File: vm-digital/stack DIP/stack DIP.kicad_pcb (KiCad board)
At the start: 2 copper layers, 20.3 x 39.1 mm, 7 parts, among them J1 Conn_01x11_Pin, J2 Conn_01x11_Pin, U1 74LS151, U2 74LS151, U3 74LS151, U4 74LS151, U5 74LS151

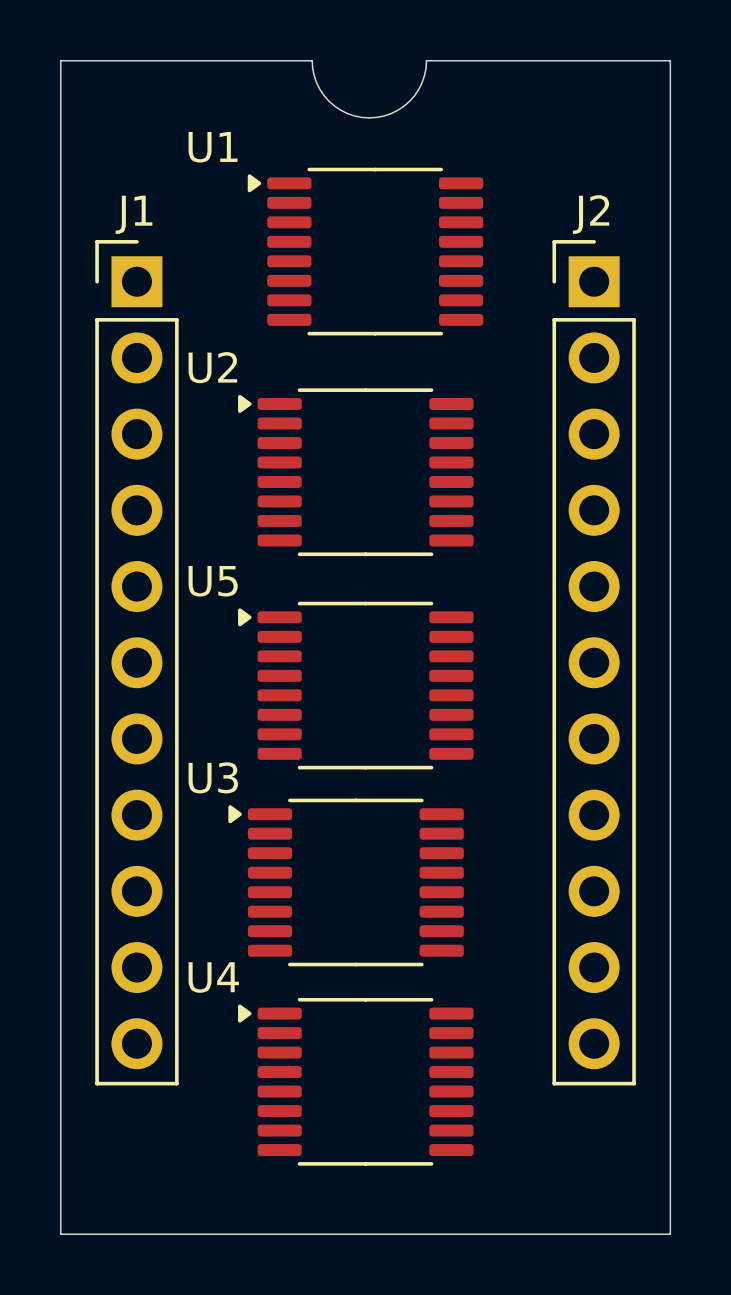
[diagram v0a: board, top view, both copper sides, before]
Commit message: stack-dip
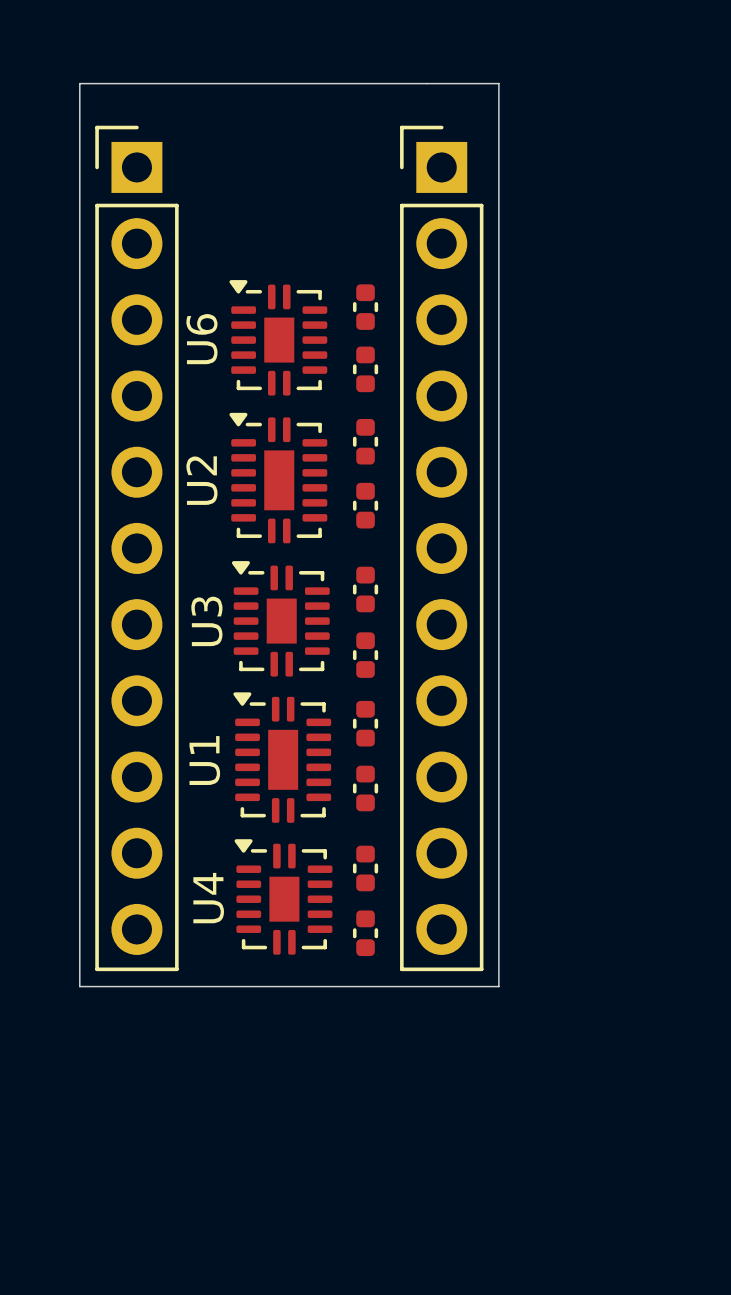
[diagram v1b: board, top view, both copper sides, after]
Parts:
- removed U5: 74LS151, Package_SO:TSSOP-16_4.4x5mm_P0.65mm
- added C1: C_Small, Capacitor_SMD:C_0402_1005Metric, F.Cu at (160.0, 68.2)
- added C10: C_Small, Capacitor_SMD:C_0402_1005Metric, F.Cu at (160.0, 77.6)
- added C2: C_Small, Capacitor_SMD:C_0402_1005Metric, F.Cu at (160.0, 70.2)
- added C3: C_Small, Capacitor_SMD:C_0402_1005Metric, F.Cu at (160.0, 72.6)
- added C4: C_Small, Capacitor_SMD:C_0402_1005Metric, F.Cu at (160.0, 74.8)
- added C5: C_Small, Capacitor_SMD:C_0402_1005Metric, F.Cu at (160.0, 89.0)
- added C6: C_Small, Capacitor_SMD:C_0402_1005Metric, F.Cu at (160.0, 86.9)
- added C7: C_Small, Capacitor_SMD:C_0402_1005Metric, F.Cu at (160.0, 84.2)
- added C8: C_Small, Capacitor_SMD:C_0402_1005Metric, F.Cu at (160.0, 82.0)
- added C9: C_Small, Capacitor_SMD:C_0402_1005Metric, F.Cu at (160.0, 79.8)
- added U6: 7408, Package_DFN_QFN:DHVQFN-14-1EP_2.5x3mm_P0.5mm_EP1x1.5mm, F.Cu at (157.1, 69.3)
- U1: value 74LS151 -> 74LS157; footprint Package_SO:TSSOP-16_4.4x5mm_P0.65mm -> Package_DFN_QFN:DHVQFN-16-1EP_2.5x3.5mm_P0.5mm_EP1x2mm
- U2: footprint Package_SO:TSSOP-16_4.4x5mm_P0.65mm -> Package_DFN_QFN:DHVQFN-16-1EP_2.5x3.5mm_P0.5mm_EP1x2mm
- U3, U4: value 74LS151 -> 74HC74; footprint Package_SO:TSSOP-16_4.4x5mm_P0.65mm -> Package_DFN_QFN:DHVQFN-14-1EP_2.5x3mm_P0.5mm_EP1x1.5mm
- moved U1 17.2 mm to (157.3, 83.2)
- moved U3 9.06 mm to (157.2, 78.6)
- moved U4 6.66 mm to (157.3, 87.9)
- moved J2 6.35 mm to (162.6, 63.5)
- moved J1 3.81 mm to (152.4, 63.5)
- moved U2 2.89 mm to (157.1, 73.9)
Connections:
- U3 pad 15: unconnected-(U3-I4-Pad15) -> (no net)
- U4 pad 15: unconnected-(U4-I4-Pad15) -> (no net)
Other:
- board size 20.3 x 39.1 mm -> 14 x 30.1 mm
- board text added: "BTM"
- board text added: "CK0"
- board text added: "CK1"
- board text added: "CK2"
- board text added: "CK3"
- board text added: "CKP"
- board text added: "DIR"
- board text added: "DS0"
- board text added: "DS1"
- board text added: "DS2"
- board text added: "DS3"
- board text added: "GND"
- board text added: "IN0"
- board text added: "IN1"
- board text added: "IN2"
- board text added: "IN3"
- board text added: "PWR"
- board text added: "Pax Instruments, Stack Module v02"
- board text added: "RST"
